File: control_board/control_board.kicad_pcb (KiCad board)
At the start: 2 copper layers, 51.2 x 76.2 mm, 41 parts, among them J1 Conn_01x08_Male, K1 G5Q-1A, Q1 Q_NPN_BEC, U1 MC78M05_TO252, U2 TSR_1-24120, U3 74LS02, U4 74LS02, U5 Conn_01x08_Male

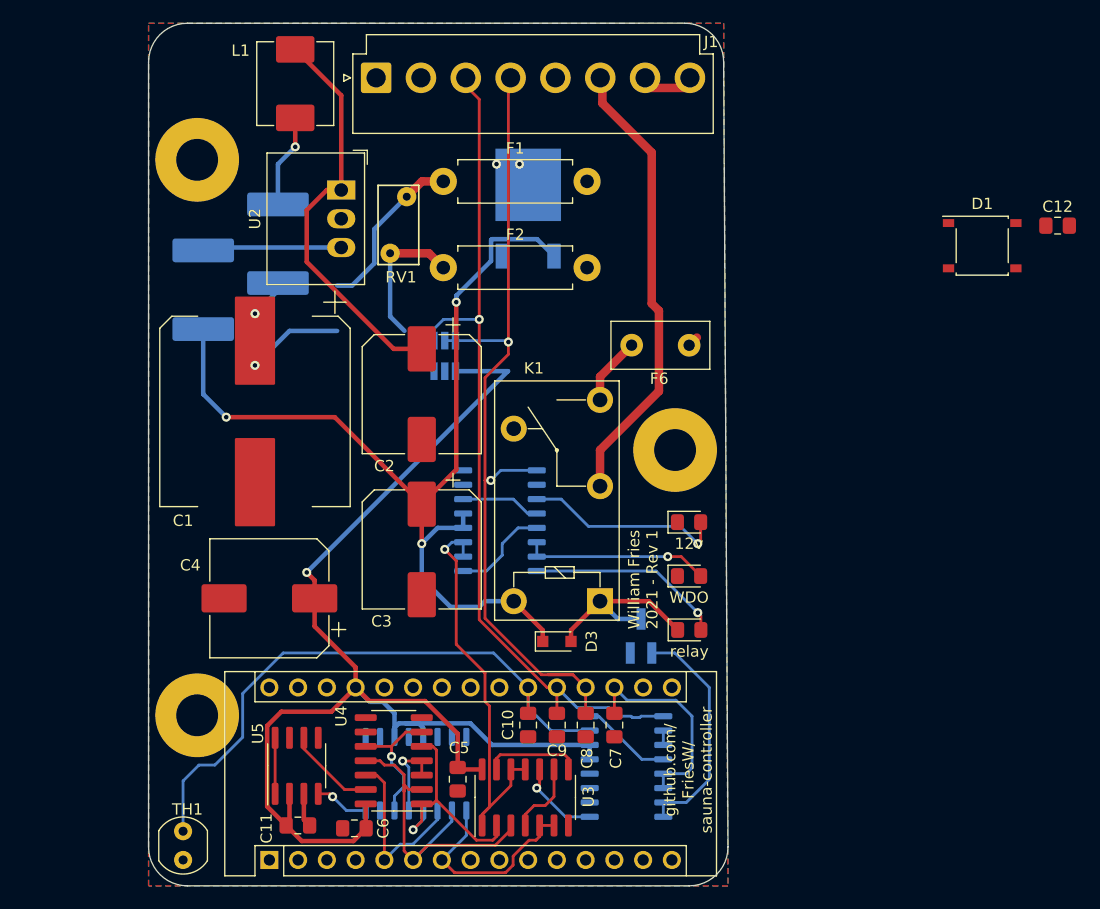
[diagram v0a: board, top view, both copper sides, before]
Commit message: Draft layout
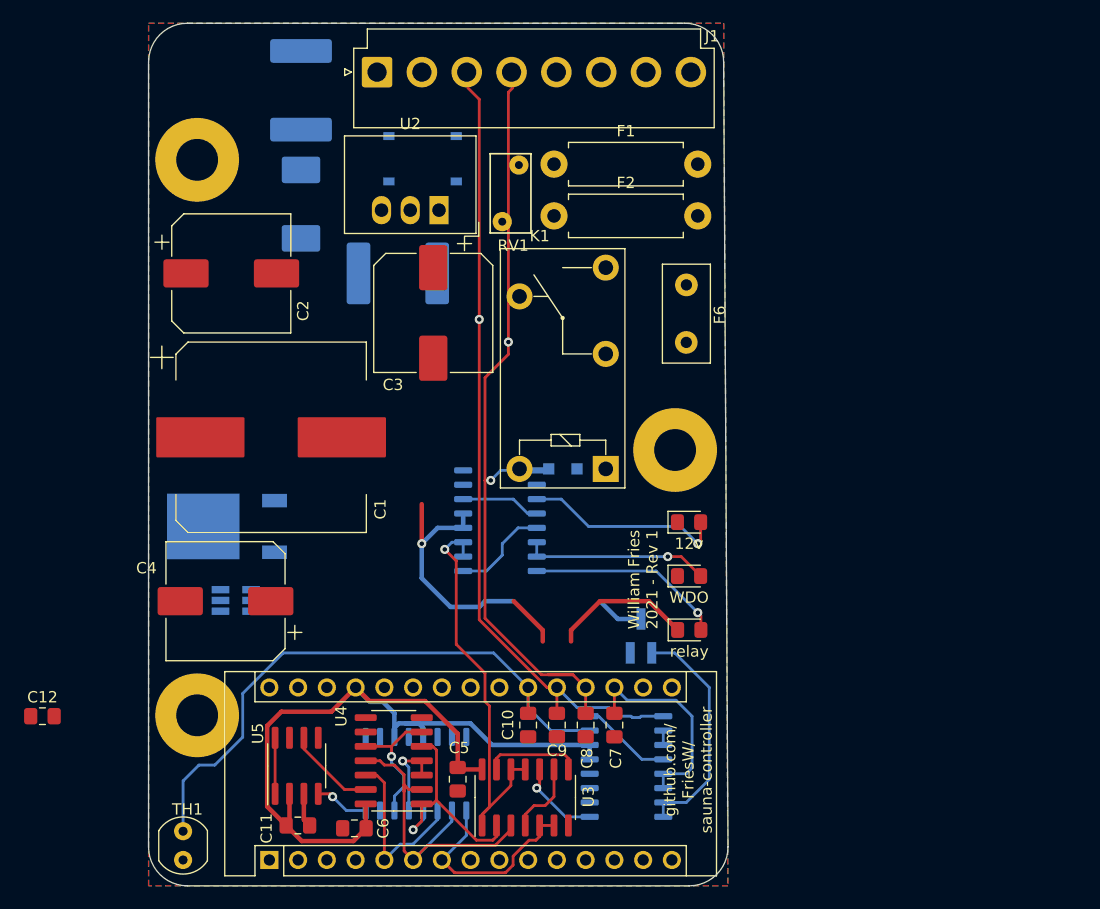
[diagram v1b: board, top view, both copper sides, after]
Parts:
- D1, D3, L1: moved to B.Cu
- moved C12 99.6 mm to (101.1, 85.3)
- moved D1 50.0 mm to (134.7, 36.1)
- moved U1 38.7 mm to (117.4, 68.6), turned to 180 degrees
- moved D2 28.4 mm to (118.2, 75.1), turned to 0 degrees
- moved C3 20.9 mm to (135.6, 49.7)
- moved C2 19.9 mm to (117.8, 46.2), turned to 0 degrees
- moved F4 17.3 mm to (132.5, 46.2), turned to 180 degrees
- moved D3 15.2 mm to (147.1, 63.5)
- moved F3 13.7 mm to (124.0, 30.1), turned to 90 degrees
- moved K1 11.7 mm to (150.9, 63.5)
- moved F2 10.8 mm to (146.3, 41.1)
- moved L1 10.7 mm to (124.0, 40.1), turned to 270 degrees
- moved RV1 10.3 mm to (141.7, 41.7)
- moved F1 9.90 mm to (146.3, 36.6)
- moved U2 8.82 mm to (136.1, 40.6), turned to 180 degrees
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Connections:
- F1 pad 1: /hv_03 -> /hv_02
- F2 pad 1: /hv_02 -> /hv_03
- RV1 pad 1: /hv_02 -> /hv_03
- RV1 pad 2: /hv_03 -> /hv_02
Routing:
- net +12V: track 87.2 -> 26.1 mm, vias 3 -> 1
- net +5V: track 119.2 -> 77.1 mm, vias 1 -> 0
- net /contactor_b: track 39.4 -> 0.00 mm
- net /hv_06: track 35.8 -> 0.00 mm
- net /hv_03: track 15.0 -> 0.00 mm
- net /hv_02: track 12.6 -> 0.00 mm
- net /hc_01: track 12.3 -> 0.00 mm
- net /hv_04: track 12.1 -> 0.00 mm, vias 2 -> 0
- net /hv_05: track 8.27 -> 0.00 mm, vias 1 -> 0
- net /sensor_a: track 77.6 -> 69.6 mm
- net /hv_07: track 5.99 -> 0.00 mm
- net /pot_a: track 74.4 -> 68.9 mm
- net GNDPWR: track 3.96 -> 0.00 mm
- net AC: track 0.97 -> 0.00 mm
- net GND: track 3.88 -> 3.00 mm, vias 2 -> 0
